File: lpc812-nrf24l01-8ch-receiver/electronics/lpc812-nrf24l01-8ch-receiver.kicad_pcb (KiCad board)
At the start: 2 copper layers, 24 parts, among them J1 CH1, J2 CH2, J3 CH3/Rx, J4 CH4/Tx, J5 CH5, J6 CH6, J7 CH7, J8 CH8, SW1 BIND/ISP, U1 MCP1703A-3302_SOT23, U2 LPC812M101JDH20, U3 NRF24L01_Breakout, Y1 16MHz

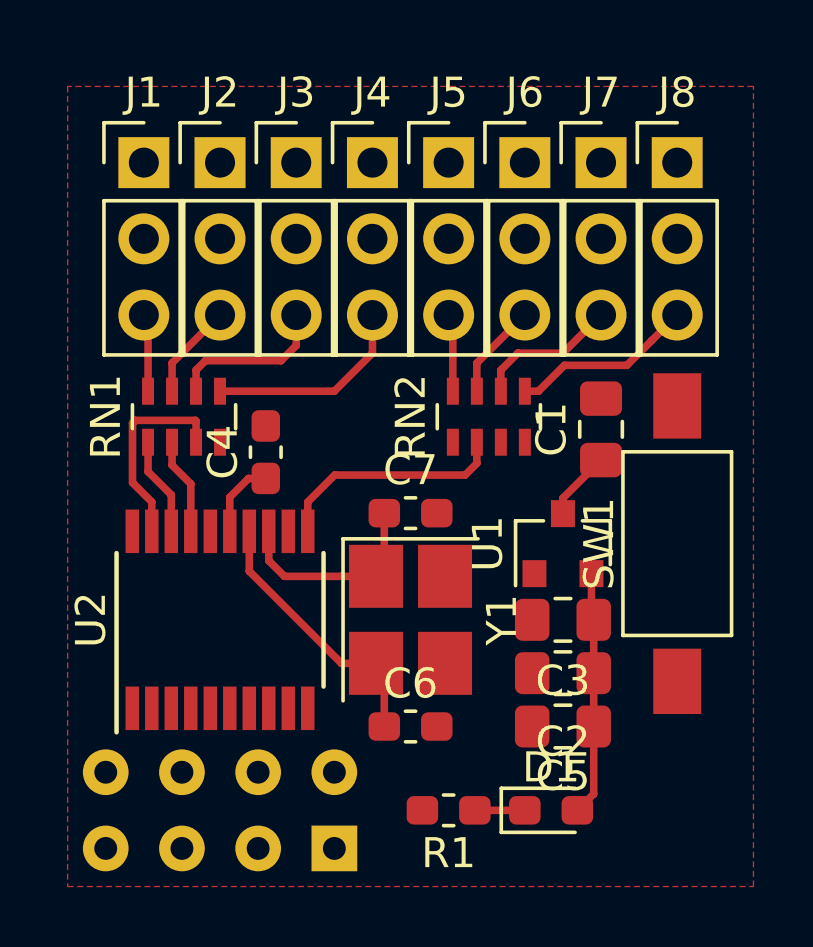
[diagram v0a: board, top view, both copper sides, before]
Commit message: Work on initial layout
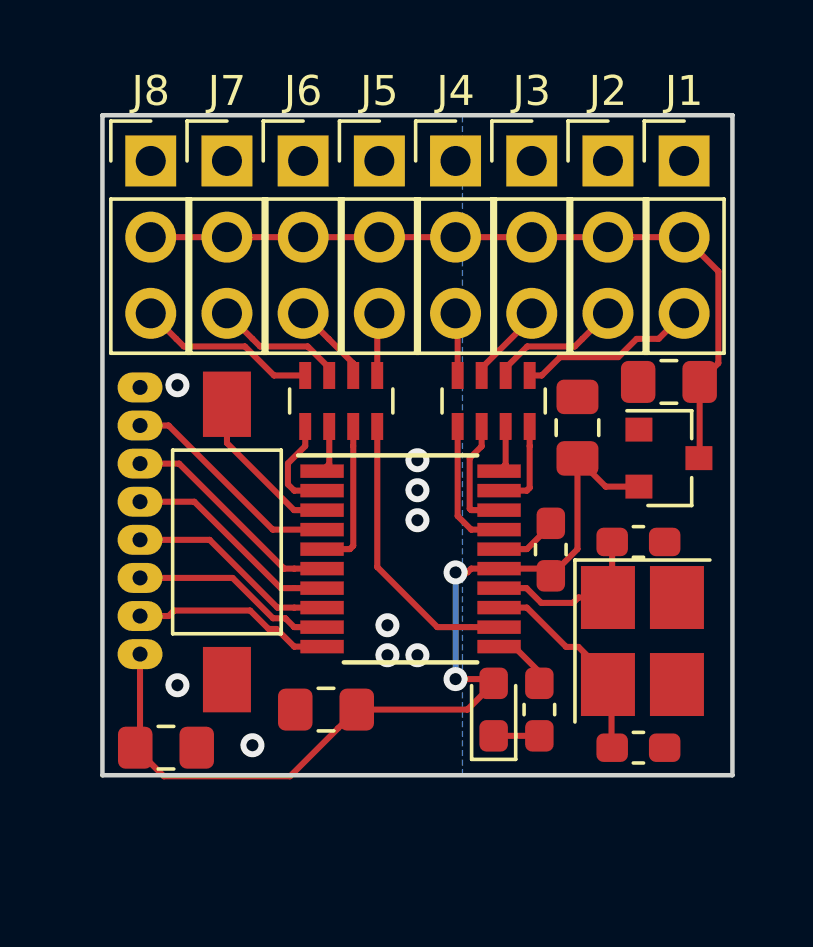
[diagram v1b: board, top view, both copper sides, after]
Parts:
- U3: footprint RF_Module:nRF24L01_Breakout -> nordic-semiconductor:nrf24l01-E01-ML01IPX
- moved J1 18.0 mm to (137.4, 68.5)
- moved J8 17.6 mm to (119.6, 68.5)
- moved SW1 15.0 mm to (122.2, 81.2), turned to 270 degrees
- moved C3 13.9 mm to (120.1, 88.1), turned to 0 degrees
- moved U3 13.0 mm to (118.6, 80.5), turned to 180 degrees
- moved J2 12.9 mm to (134.8, 68.5)
- moved J7 12.5 mm to (122.2, 68.5)
- moved RN1 10.3 mm to (131.0, 76.5)
- moved C4 10.0 mm to (132.9, 81.5)
- moved C2 8.20 mm to (133.8, 77.4), turned to 90 degrees
- moved C5 7.92 mm to (125.5, 86.8)
- moved J3 7.85 mm to (132.3, 68.5)
- moved Y1 7.76 mm to (136.0, 84.5)
- moved C7 7.66 mm to (135.9, 81.2)
- moved C6 7.63 mm to (135.9, 88.1)
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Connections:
- C6 pad 1: /XTALIN -> /XTALOUT
- C7 pad 1: /XTALOUT -> /XTALIN
- RN1 pad 1: /CH1 -> /CH4
- RN1 pad 2: /CH2 -> /CH3
- RN1 pad 3: /CH3-Rx -> /CH2
- RN1 pad 4: /CH4-Tx -> /CH1-Rx
- RN1 pad 5: Net-(J4-Pad3) -> Net-(J1-Pad3)
- RN1 pad 6: Net-(J3-Pad3) -> Net-(J2-Pad3)
- RN1 pad 7: Net-(J2-Pad3) -> Net-(J3-Pad3)
- RN1 pad 8: Net-(J1-Pad3) -> Net-(J4-Pad3)
- RN2 pad 1: /CH5 -> /CH8
- RN2 pad 2: /CH6 -> /CH7
- RN2 pad 3: /CH7 -> /CH6-Tx
- RN2 pad 4: /CH8 -> /CH5
- RN2 pad 5: Net-(J8-Pad3) -> Net-(J5-Pad3)
- RN2 pad 6: Net-(J7-Pad3) -> Net-(J6-Pad3)
- RN2 pad 7: Net-(J6-Pad3) -> Net-(J7-Pad3)
- RN2 pad 8: Net-(J5-Pad3) -> Net-(J8-Pad3)
- U2 pad 1: /CH8 -> /CH7
- U2 pad 10: /CH7 -> /CE
- U2 pad 11: /CH6 -> /LED
- U2 pad 12: /SCK -> /CH5
- U2 pad 17: /CH2 -> /CH4
- U2 pad 18: /CH1 -> /CH3
- U2 pad 19: /CH3-Rx -> /CH1-Rx
- U2 pad 2: /CE -> /CH8
- U2 pad 20: /CH5 -> /CH2
- U2 pad 4: /LED -> /IRQ
- U2 pad 5: /CH4-Tx -> /CH6-Tx
- U2 pad 6: /CSN -> /MISO
- U2 pad 8: /MISO -> /SCK
- U2 pad 9: /IRQ -> /CSN
- Y1 pad 1: /XTALOUT -> /XTALIN
- Y1 pad 2: /XTALIN -> /XTALOUT
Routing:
- net VDD: track 2.31 -> 25.9 mm
- net VCC: track 10.7 -> 31.7 mm, vias 0 -> 2
- net /CH5: track 0.00 -> 9.57 mm
- net /CH6: track 7.85 -> 0.00 mm
- net /MISO: track 0.00 -> 7.52 mm
- net /MOSI: track 0.00 -> 7.26 mm
- net /IRQ: track 0.00 -> 7.15 mm
- net /SCK: track 0.00 -> 7.00 mm
- net /CSN: track 0.00 -> 6.75 mm
- net /CH3-Rx: track 6.74 -> 0.00 mm
- net /CE: track 0.00 -> 6.64 mm
- net /BIND-ISP: track 0.00 -> 5.39 mm
- net /CH6-Tx: track 0.00 -> 5.06 mm
- net Net-(J4-Pad3): track 6.88 -> 2.10 mm
- net /CH4: track 0.00 -> 4.55 mm
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- added copper zone on B.Cu, net GND
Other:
- board outline added: 21 x 22 mm
- net class Default: trace_width 0.254 -> 0.2032
